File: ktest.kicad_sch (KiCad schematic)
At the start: 41 parts, among them J1 Conn_01x03_Pin, U2 ATmega8-16P

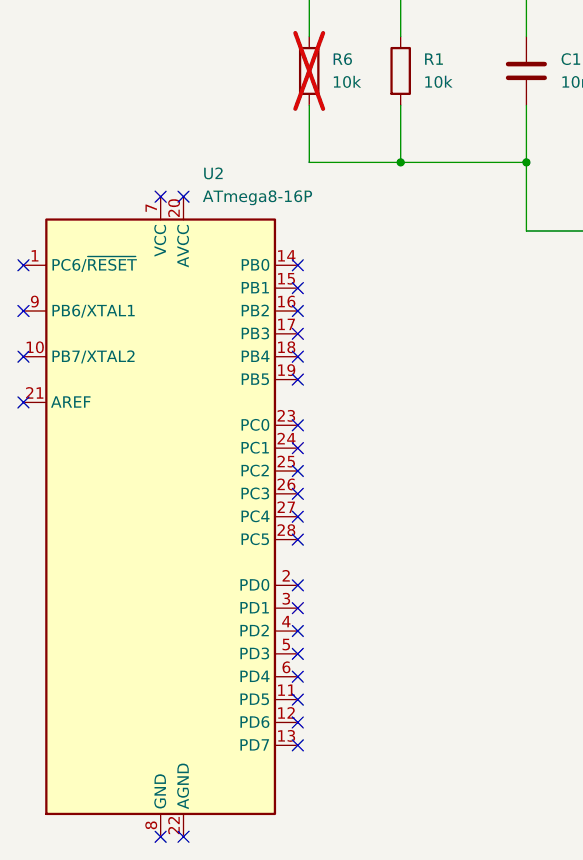
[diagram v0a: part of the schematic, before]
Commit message: merging scripts
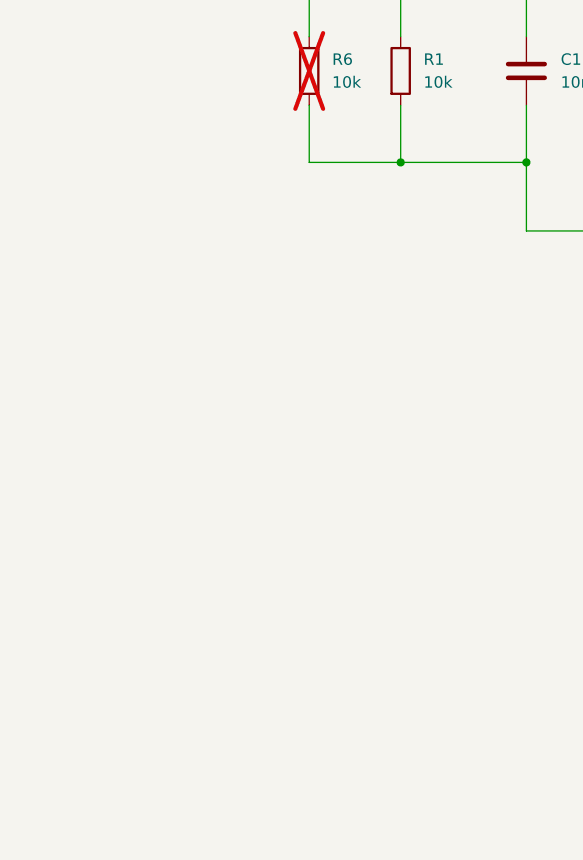
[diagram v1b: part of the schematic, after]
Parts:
- removed U2: ATmega8-16P, Package_DIP:DIP-28_W7.62mm, symbol MCU_Microchip_ATmega:ATmega8-16P
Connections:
- no-connect marks 28 -> 0
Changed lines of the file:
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@@
 		(color 0 0 0 0)
-	)
-	(no_connect
-		(at 64.77 148.59)
-	)
-	(no_connect
-		(at 34.29 123.19)
-	)
-	(no_connect
-		(at 64.77 123.19)
-	)
-	(no_connect
-		(at 64.77 158.75)
-	)
-	(no_connect
-		(at 34.29 128.27)
-	)
-	(no_connect
-		(at 64.77 166.37)
-	)
-	(no_connect
-		(at 64.77 130.81)
-	)
-	(no_connect
-		(at 64.77 173.99)
-	)
-	(no_connect
-		(at 34.29 138.43)
-	)
-	(no_connect
-		(at 64.77 161.29)
-	)
-	(no_connect
-		(at 64.77 135.89)
-	)
-	(no_connect
-		(at 64.77 153.67)
-	)
-	(no_connect
-		(at 64.77 163.83)
-	)
-	(no_connect
-		(at 64.77 176.53)
-	)
-	(no_connect
-		(at 52.07 115.57)
-	)
-	(no_connect
-		(at 64.77 128.27)
-	)
-	(no_connect
-		(at 49.53 186.69)
-	)
-	(no_connect
-		(at 64.77 151.13)
-	)
-	(no_connect
-		(at 34.29 133.35)
-	)
-	(no_connect
-		(at 64.77 140.97)
-	)
-	(no_connect
-		(at 64.77 125.73)
-	)
-	(no_connect
-		(at 64.77 143.51)
-	)
-	(no_connect
-		(at 52.07 186.69)
-	)
-	(no_connect
-		(at 64.77 146.05)
-	)
-	(no_connect
-		(at 64.77 168.91)
-	)
-	(no_connect
-		(at 64.77 133.35)
-	)
-	(no_connect
-		(at 64.77 171.45)
-	)
-	(no_connect
-		(at 49.53 115.57)
 	)
 	(wire
@@
 					(unit 1)
 				)
-			)
-		)
-	)
-	(symbol
-		(lib_id "MCU_Microchip_ATmega:ATmega8-16P")
-		(at 49.53 151.13 0)
-		(unit 1)
-		(body_style 1)
-		(exclude_from_sim no)
-		(in_bom yes)
-		(on_board yes)
-		(in_pos_files yes)
-		(dnp no)
-		(fields_autoplaced yes)
-		(property "Reference" "U2"
-			(at 54.2133 113.03 0)
-			(show_name no)
-			(do_not_autoplace no)
-			(effects
-				(font
-					(size 1.27 1.27)
-				)
-				(justify left)
-			)
-		)
-		(property "Value" "ATmega8-16P"
-			(at 54.2133 115.57 0)
-			(show_name no)
-			(do_not_autoplace no)
-			(effects
-				(font
-					(size 1.27 1.27)
-				)
-				(justify left)
-			)
-		)
-		(property "Footprint" "Package_DIP:DIP-28_W7.62mm"
-			(at 49.53 151.13 0)
-			(hide yes)
-			(show_name no)
-			(do_not_autoplace no)
-			(effects
-				(font
-					(size 1.27 1.27)
-					(italic yes)
-				)
-			)
-		)
-		(property "Datasheet" "http://ww1.microchip.com/downloads/en/DeviceDoc/atmel-2486-8-bit-avr-microcontroller-atmega8_l_datasheet.pdf"
-			(at 49.53 151.13 0)
-			(hide yes)
-			(show_name no)
-			(do_not_autoplace no)
-			(effects
-				(font
-					(size 1.27 1.27)
-				)
-			)
-		)
-		(property "Description" "16MHz, 8kB Flash, 1kB SRAM, 512B EEPROM, DIP-28"
-			(at 49.53 151.13 0)
-			(hide yes)
-			(show_name no)
-			(do_not_autoplace no)
-			(effects
-				(font
-					(size 1.27 1.27)
-				)
-			)
-		)
-		(pin "13"
-		)
-		(pin "15"
-		)
-		(pin "2"
-		)
-		(pin "4"
-		)
-		(pin "12"
-		)
-		(pin "14"
-		)
-		(pin "22"
-		)
-		(pin "23"
-		)
-		(pin "16"
-		)
-		(pin "18"
-		)
-		(pin "9"
-		)
-		(pin "5"
-		)
-		(pin "19"
-		)
-		(pin "20"
-		)
-		(pin "10"
-		)
-		(pin "8"
-		)
-		(pin "6"
-		)
-		(pin "11"
-		)
-		(pin "21"
-		)
-		(pin "7"
-		)
-		(pin "27"
-		)
-		(pin "28"
-		)
-		(pin "25"
-		)
-		(pin "26"
-		)
-		(pin "3"
-		)
-		(pin "17"
-		)
-		(pin "1"
-		)
-		(pin "24"
-		)
-		(instances
-			(project "ktest"
-				(path "/f14ff7c3-fe34-4697-84b8-3cc06a5a3565"
-					(reference "U2")
-					(unit 1)
-				)
